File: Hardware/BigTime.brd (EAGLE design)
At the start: 25.4 x 25.4 mm, 21 parts, among them U2 ATMEGA328P_TQFP, Y1 32.768kHz

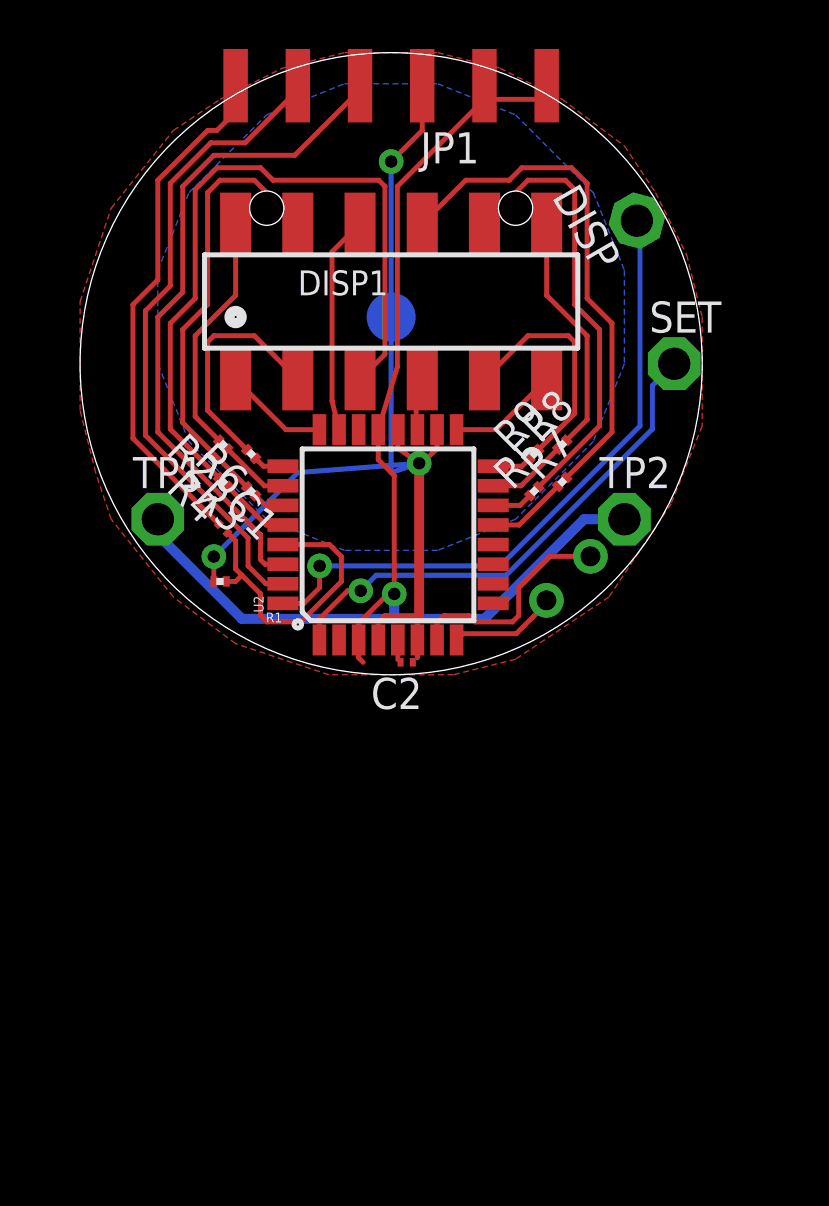
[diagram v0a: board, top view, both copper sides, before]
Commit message: fit
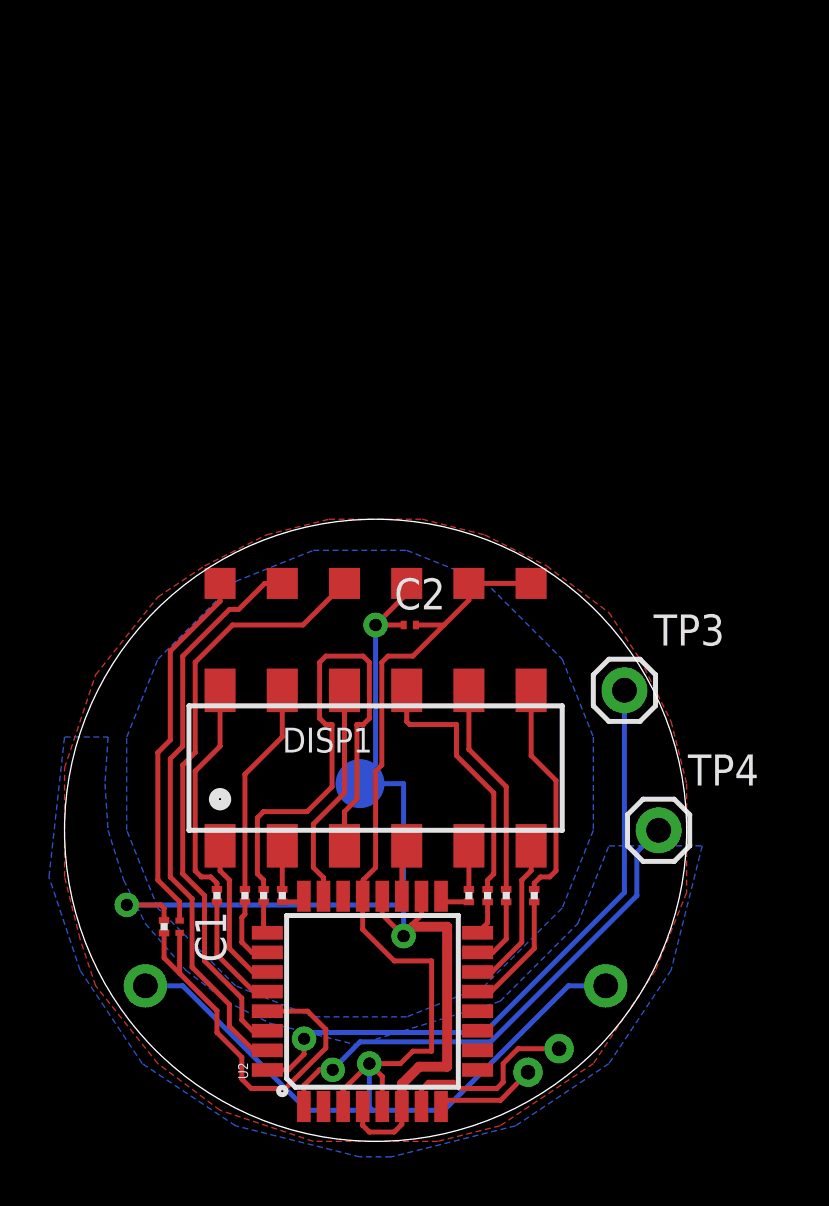
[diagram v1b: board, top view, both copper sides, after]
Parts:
- removed DISP, SET: TPPAD1-13, testpad:P1-13
- removed TP1, TP2: PTR1PAD1-13, testpad:P1-13
- removed U$2: CREATIVE_COMMONS, SparkFun:CREATIVE_COMMONS
- removed VCC: TPTP20R, testpad:TP20R
- added BAT+: TPTP20R, testpad:TP20R
- added TP3, TP4: (no value), SparkFun-Connectors:1X01
- added TP5, TP6: (no value), adafruit:1X01-CLEANBIG
- DISP1: device SparkFun-Displays:DIL12_SM -> BigTime:DIL12_SM
- JP1: value (none) -> FTDI_DEVICERA_SMT; device SparkFun-Connectors:1X06-SMD -> BigTime:FTDI_DEVICE_RA_SMT
- Y1: device crystal:TC26H -> BigTime:TC26H
- moved Y1 19.8 mm to (20.8, 7.11), turned to 270 degrees
- moved DISP1 19.1 mm to (14.6, 19.1)
- moved U2 19.1 mm to (14.5, 9.53)
- moved R8 18.5 mm to (21.1, 13.8), turned to 90 degrees
- moved R2 18.4 mm to (8.13, 13.8), turned to 90 degrees
- moved R9 18.2 mm to (18.4, 13.8), turned to 90 degrees
- moved R6 18.1 mm to (10.8, 13.8), turned to 90 degrees
- moved R7 17.2 mm to (19.2, 13.8), turned to 90 degrees
- moved R4 17.0 mm to (10.0, 13.8), turned to 90 degrees
- moved R5 16.5 mm to (19.9, 13.8), turned to 90 degrees
- moved R3 16.5 mm to (9.27, 13.8), turned to 90 degrees
- moved C1 16.4 mm to (6.60, 12.6), turned to 270 degrees
- moved JP1 15.3 mm to (14.6, 26.7)
- moved R1 14.3 mm to (5.97, 12.6), turned to 90 degrees
- moved C2 1.53 mm to (16.0, 24.9), turned to 0 degrees
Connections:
- net A: now also U2.28; no longer U2.26
- net B: now also U2.26; no longer U2.27
- net BTN: now also TP3.1; no longer DISP.TP
- net C: now also U2.25; no longer U2.28
- net D: now also U2.15; no longer U2.14
- net DIG1: now also U2.27; no longer U2.24
- net DIG4: now also U2.14; no longer U2.17
- net DP: now also U2.17; no longer U2.16
- net E: now also U2.24; no longer U2.25
- net F: now also U2.16; no longer U2.13
- net G: now also U2.13; no longer U2.15
- net GND: now also TP5.1, TP6.1; no longer TP1.TP, TP2.TP
- net RXI: now also JP1.2; no longer JP1.3
- net SET: now also TP4.1; no longer SET.TP
- net TXO: now also JP1.3; no longer JP1.2
- net VCC: now also BAT+.TP; no longer VCC.TP
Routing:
- net N$9: track 21.1 -> 10.8 mm
- net N$7: track 18.2 -> 8.76 mm
- net N$5: track 18.1 -> 8.76 mm
- net N$8: track 9.58 -> 1.78 mm
- net N$11: track 9.53 -> 1.78 mm
- net N$6: track 29.7 -> 22.3 mm
- net VCC: track 42.4 -> 49.4 mm
- net N$3: track 21.3 -> 15.4 mm
- net GND: track 53.9 -> 59.1 mm
- net RST: track 12.4 -> 16.7 mm
- net RXI: track 27.4 -> 24.5 mm
- net TXO: track 26.5 -> 23.6 mm
- net DIG1: track 4.28 -> 6.30 mm
- net A: track 2.88 -> 4.84 mm
- net DIG4: track 4.53 -> 6.40 mm
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- added copper zone on layer 16, net GND
